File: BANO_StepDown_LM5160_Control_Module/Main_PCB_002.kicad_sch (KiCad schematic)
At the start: 73 parts, among them U1 SI7489DP-T1-E3, U2 STM32G031G8Ux, U3 LM5160ADNTR, U4 LM5160ADNTR, U5 INA193

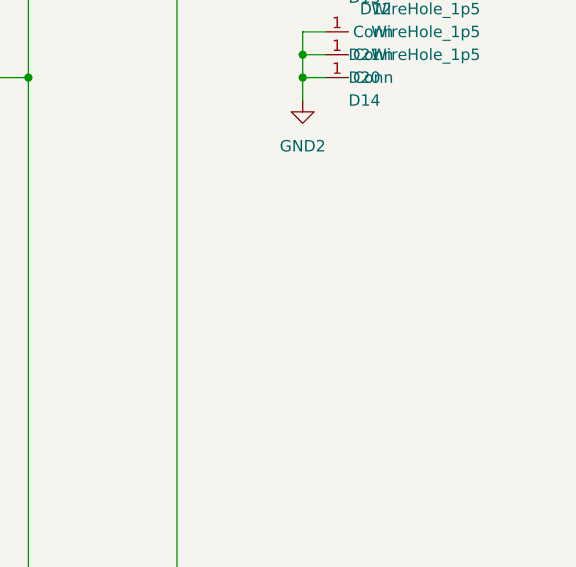
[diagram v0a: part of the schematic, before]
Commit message: PCB work 6
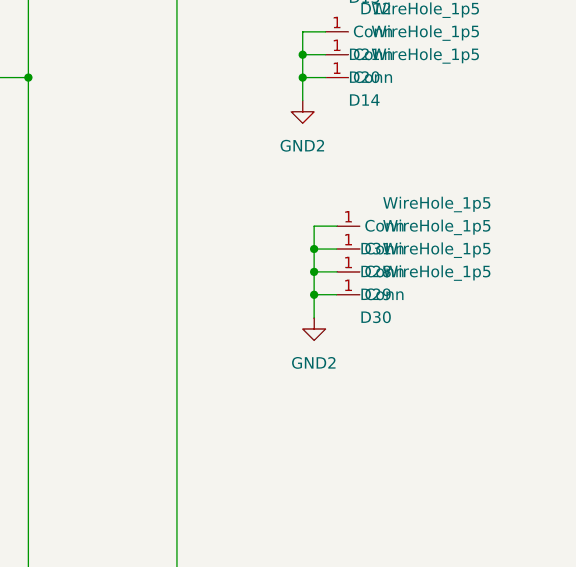
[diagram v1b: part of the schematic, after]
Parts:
- added D28, D29, D30, D31: WireHole_1p5, Wire_holes:WireHole_2p0, symbol Connectors_for_Wire:WireHole_1p5
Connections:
- net GND2: now also D28.1 (Conn), D29.1 (Conn), D30.1 (Conn), D31.1 (Conn)
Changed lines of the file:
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@@
   (junction (at 492.76 248.92) (diameter 0) (color 0 0 0 0)
   )
+  (junction (at 553.72 173.99) (diameter 0) (color 0 0 0 0)
+  )
   (junction (at 411.48 157.48) (diameter 0) (color 0 0 0 0)
   )
   (junction (at 300.99 144.78) (diameter 0) (color 0 0 0 0)
   )
+  (junction (at 553.72 176.53) (diameter 0) (color 0 0 0 0)
+  )
   (junction (at 491.49 172.72) (diameter 0) (color 0 0 0 0)
   )
@@
   (junction (at 387.35 144.78) (diameter 0) (color 0 0 0 0)
   )
+  (junction (at 553.72 179.07) (diameter 0) (color 0 0 0 0)
+  )
   (junction (at 234.95 160.02) (diameter 0) (color 0 0 0 0)
   )
@@
     (stroke (width 0) (type default))
   )
+  (wire (pts (xy 556.26 171.45) (xy 553.72 171.45))
+    (stroke (width 0) (type default))
+  )
   (wire (pts (xy 491.49 160.02) (xy 491.49 154.94))
     (stroke (width 0) (type default))
@@
     (stroke (width 0) (type default))
   )
+  (wire (pts (xy 553.72 179.07) (xy 553.72 181.61))
+    (stroke (width 0) (type default))
+  )
+  (wire (pts (xy 553.72 176.53) (xy 553.72 179.07))
+    (stroke (width 0) (type default))
+  )
   (wire (pts (xy 471.17 240.03) (xy 471.17 242.57))
     (stroke (width 0) (type default))
@@
     (stroke (width 0) (type default))
   )
+  (wire (pts (xy 556.26 179.07) (xy 553.72 179.07))
+    (stroke (width 0) (type default))
+  )
   (wire (pts (xy 441.96 252.73) (xy 448.31 252.73))
     (stroke (width 0) (type default))
@@
     (stroke (width 0) (type default))
   )
+  (wire (pts (xy 556.26 176.53) (xy 553.72 176.53))
+    (stroke (width 0) (type default))
+  )
   (wire (pts (xy 457.2 144.78) (xy 462.28 144.78))
     (stroke (width 0) (type default))
@@
     (stroke (width 0) (type default))
   )
+  (wire (pts (xy 556.26 173.99) (xy 553.72 173.99))
+    (stroke (width 0) (type default))
+  )
   (wire (pts (xy 411.48 149.86) (xy 411.48 157.48))
     (stroke (width 0) (type default))
@@
     (stroke (width 0) (type default))
   )
+  (wire (pts (xy 553.72 171.45) (xy 553.72 173.99))
+    (stroke (width 0) (type default))
+  )
   (wire (pts (xy 504.19 259.08) (xy 504.19 260.35))
     (stroke (width 0) (type default))
@@
   )
   (wire (pts (xy 471.17 250.19) (xy 471.17 252.73))
+    (stroke (width 0) (type default))
+  )
+  (wire (pts (xy 553.72 173.99) (xy 553.72 176.53))
     (stroke (width 0) (type default))
   )
@@
     )
   )
+  (symbol (lib_id "Connectors_for_Wire:WireHole_1p5") (at 556.26 179.07 0) (unit 1)
+    (in_bom yes) (on_board yes) (dnp no)
+    (property "Reference" "D30" (at 558.8 181.61 0)
+      (effects (font (size 1.27 1.27)) (justify left))
+    )
+    (property "Value" "WireHole_1p5" (at 561.34 176.53 0)
+      (effects (font (size 1.27 1.27)) (justify left))
+    )
+    (property "Footprint" "Wire_holes:WireHole_2p0" (at 556.26 180.34 0)
+      (effects (font (size 1.27 1.27)) hide)
+    )
+    (property "Datasheet" "" (at 556.26 180.34 0)
+      (effects (font (size 1.27 1.27)) hide)
+    )
+    (pin "1")
+    (instances
+      (project "Main_PCB_002"
+        (path "/68e09be7-3bbc-4443-a838-209ce20b2bef"
+          (reference "D30") (unit 1)
+        )
+      )
+    )
+  )
   (symbol (lib_id "Connectors_for_Wire:WireHole_1p5") (at 554.99 140.97 0) (unit 1)
     (in_bom yes) (on_board yes) (dnp no)
@@
         (path "/68e09be7-3bbc-4443-a838-209ce20b2bef"
           (reference "#PWR016") (unit 1)
+        )
+      )
+    )
+  )
+  (symbol (lib_id "Connectors_for_Wire:WireHole_1p5") (at 556.26 176.53 0) (unit 1)
+    (in_bom yes) (on_board yes) (dnp no)
+    (property "Reference" "D29" (at 558.8 179.07 0)
+      (effects (font (size 1.27 1.27)) (justify left))
+    )
+    (property "Value" "WireHole_1p5" (at 561.34 173.99 0)
+      (effects (font (size 1.27 1.27)) (justify left))
+    )
+    (property "Footprint" "Wire_holes:WireHole_2p0" (at 556.26 177.8 0)
+      (effects (font (size 1.27 1.27)) hide)
+    )
+    (property "Datasheet" "" (at 556.26 177.8 0)
+      (effects (font (size 1.27 1.27)) hide)
+    )
+    (pin "1")
+    (instances
+      (project "Main_PCB_002"
+        (path "/68e09be7-3bbc-4443-a838-209ce20b2bef"
+          (reference "D29") (unit 1)
         )
       )
@@
     )
   )
+  (symbol (lib_id "power:GND2") (at 553.72 181.61 0) (unit 1)
+    (in_bom yes) (on_board yes) (dnp no) (fields_autoplaced)
+    (property "Reference" "#PWR030" (at 553.72 187.96 0)
+      (effects (font (size 1.27 1.27)) hide)
+    )
+    (property "Value" "GND2" (at 553.72 186.69 0)
+      (effects (font (size 1.27 1.27)))
+    )
+    (property "Footprint" "" (at 553.72 181.61 0)
+      (effects (font (size 1.27 1.27)) hide)
+    )
+    (property "Datasheet" "" (at 553.72 181.61 0)
+      (effects (font (size 1.27 1.27)) hide)
+    )
+    (pin "1")
+    (instances
+      (project "Main_PCB_002"
+        (path "/68e09be7-3bbc-4443-a838-209ce20b2bef"
+          (reference "#PWR030") (unit 1)
+        )
+      )
+    )
+  )
   (symbol (lib_id "Device:C") (at 229.87 166.37 0) (unit 1)
     (in_bom yes) (on_board yes) (dnp no)
@@
         )
       )
+    )
+  )
+  (symbol (lib_id "Connectors_for_Wire:WireHole_1p5") (at 556.26 171.45 0) (unit 1)
+    (in_bom yes) (on_board yes) (dnp no)
+    (property "Reference" "D31" (at 558.8 173.99 0)
+      (effects (font (size 1.27 1.27)) (justify left))
+    )
+    (property "Value" "WireHole_1p5" (at 561.34 168.91 0)
+      (effects (font (size 1.27 1.27)) (justify left))
+    )
+    (property "Footprint" "Wire_holes:WireHole_2p0" (at 556.26 172.72 0)
+      (effects (font (size 1.27 1.27)) hide)
+    )
+    (property "Datasheet" "" (at 556.26 172.72 0)
+      (effects (font (size 1.27 1.27)) hide)
+    )
+    (pin "1")
+    (instances
+      (project "Main_PCB_002"
+        (path "/68e09be7-3bbc-4443-a838-209ce20b2bef"
+          (reference "D31") (unit 1)
+        )
+      )
+    )
+  )
+  (symbol (lib_id "Connectors_for_Wire:WireHole_1p5") (at 556.26 173.99 0) (unit 1)
+    (in_bom yes) (on_board yes) (dnp no)
+    (property "Reference" "D28" (at 558.8 176.53 0)
+      (effects (font (size 1.27 1.27)) (justify left))
+    )
+    (property "Value" "WireHole_1p5" (at 561.34 171.45 0)
+      (effects (font (size 1.27 1.27)) (justify left))
+    )
+    (property "Footprint" "Wire_holes:WireHole_2p0" (at 556.26 175.26 0)
+      (effects (font (size 1.27 1.27)) hide)
+    )
+    (property "Datasheet" "" (at 556.26 175.26 0)
+      (effects (font (size 1.27 1.27)) hide)
+    )
+    (pin "1")
+    (instances
+      (project "Main_PCB_002"
+        (path "/68e09be7-3bbc-4443-a838-209ce20b2bef"
+          (reference "D28") (unit 1)
+        )
+      )
